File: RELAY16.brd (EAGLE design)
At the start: 118.1 x 69.8 mm, 118 parts, among them J1 Analog, J2 POWER, J3 Digital_0_7, J4 M100.1, J5 ICSPPTH, J6 Digital_0_7, J7 PWR SELECT, J8 Digital_0_7, J9 Digital_0_7, Q1 2N7002, Q10 2N7002, Q11 2N7002, Q12 2N7002, Q13 2N7002, Q14 2N7002, Q15 2N7002, Q16 2N7002, Q2 2N7002, Q3 2N7002, Q4 2N7002, Q5 2N7002, Q6 2N7002, Q7 2N7002, Q8 2N7002, Q9 2N7002

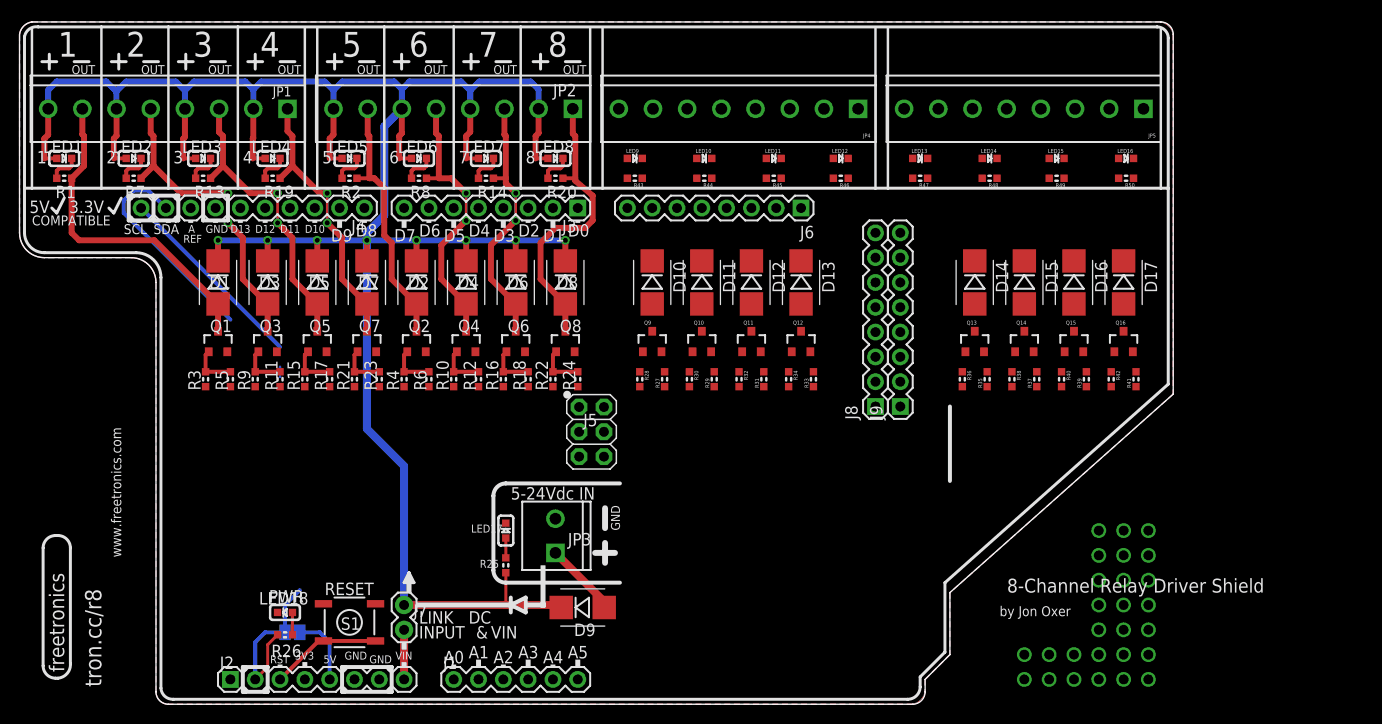
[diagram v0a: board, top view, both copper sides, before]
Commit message: Rough draft
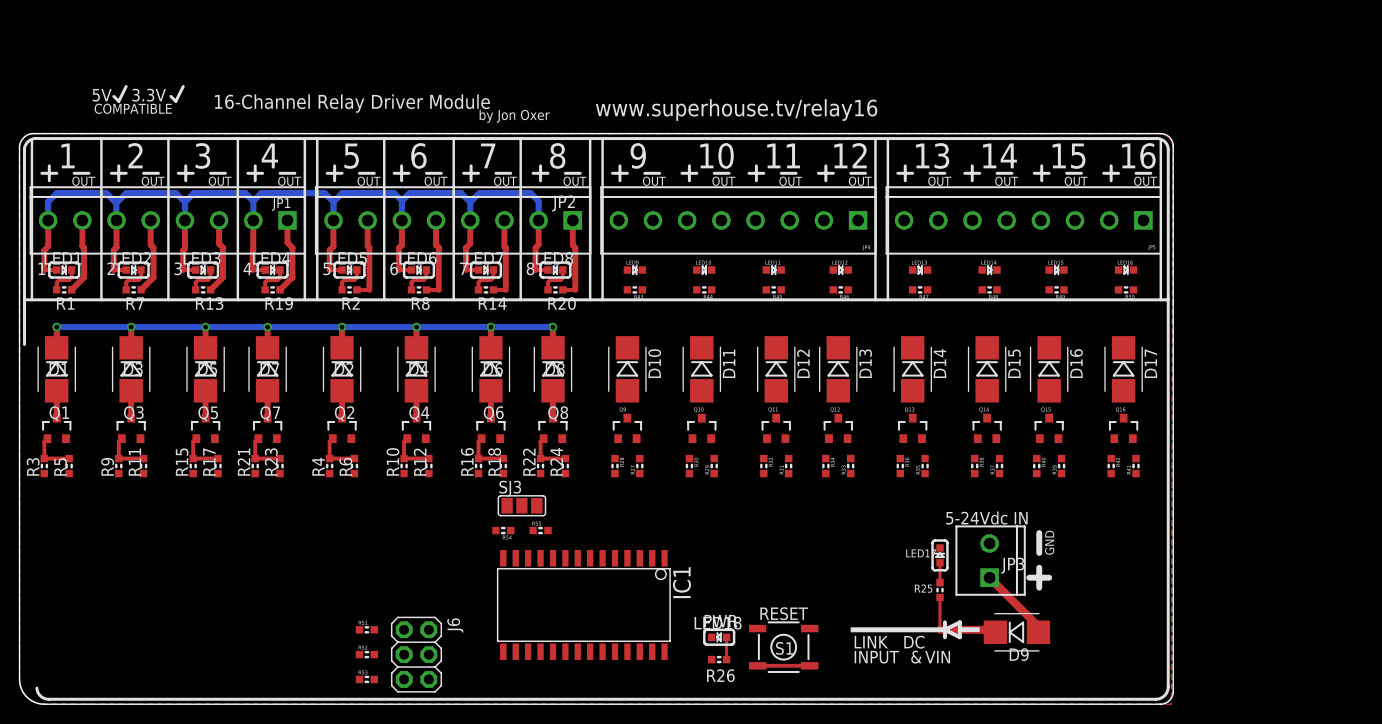
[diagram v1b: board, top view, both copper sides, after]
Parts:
- removed J1: Analog, freetronics:1X06
- removed J2: POWER, freetronics:1X08
- removed J3, J8, J9: Digital_0_7, freetronics:1X08
- removed J4: M100.1, freetronics-original:1X10
- removed J5: ICSPPTH, freetronics-jon:2X03PTH
- removed J7: PWR SELECT, SparkFun:1X02
- removed SJ4: (no value), freetronics-jon:SJ
- added IC1: MCP23017SO, microchip:SO28W
- added R51, R52, R53: 10K, freetronics-master-v1:0603
- added R54, R55: 4K7, freetronics-master-v1:0603
- added SJ3: (no value), freetronics-master-v1.1:SJ_2
- J6: value Digital_0_7 -> (none); device freetronics:1X08 -> freetronics-master-v1.1:2X03
- moved J6 60.3 mm to (40.6, 5.08), turned to 270 degrees
- moved D9 44.5 mm to (102.1, 7.37)
- moved LED18 44.5 mm to (71.6, 6.86)
- moved R26 44.5 mm to (71.6, 4.57)
- moved S1 44.5 mm to (78.2, 5.84)
- moved JP3 44.5 mm to (99.3, 13.0)
- moved LED17 44.5 mm to (94.2, 15.2)
- moved R25 44.5 mm to (94.2, 11.7)
- moved D1 18.8 mm to (3.81, 34.3)
- moved Q1 18.8 mm to (3.81, 28.2)
- moved R3 18.8 mm to (2.54, 24.4)
- moved R5 18.8 mm to (5.08, 24.4)
- moved Q3 16.6 mm to (11.4, 28.2)
- moved D3 16.6 mm to (11.4, 34.3)
- moved R11 16.6 mm to (12.7, 24.4)
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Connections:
- removed net 3V3: J2.4
- removed net 5V: J2.5, SJ4.2
- removed net A0: J1.1
- removed net A1: J1.2
- removed net A2: J1.3
- removed net A3: J1.4
- removed net A4_SDA: J1.5
- removed net A5_SCL: J1.6
- removed net AREF: J4.8
- removed net D0_RX: J3.1
- removed net D10: J4.3
- removed net D11_MOSI: J4.4
- removed net D12_MISO: J4.5
- removed net D13_SCK: J4.6
- removed net D1_TX: J3.2
- removed net D2: J3.3
- removed net D22: J8.8
- removed net D23: J9.8
- removed net D24: J8.7
- removed net D25: J9.7
- removed net D26: J8.6
- removed net D27: J9.6
- removed net D28: J8.5
- removed net D29: J9.5
- removed net D3: J3.4
- removed net D30: J8.4
- removed net D31: J9.4
- removed net D32: J8.3
- removed net D33: J9.3
- removed net D34: J8.2
- removed net D35: J9.2
- removed net D36: J8.1
- removed net D37: J9.1
- removed net D4: J3.5
- removed net D5: J3.6
- removed net D6: J3.7
- removed net D7: J3.8
- removed net D8: J4.1
- removed net D9: J4.2
- removed net N$71: J6.8
- removed net N$72: J6.7
- removed net N$73: J6.6
- removed net N$74: J6.5
- removed net N$75: J6.4
- removed net N$76: J6.3
- removed net N$77: J6.2
- removed net N$78: J6.1
- removed net NC: J2.1
- removed net R3_SCL: J4.10
- removed net R3_SDA: J4.9
- removed net VIN: J2.8, J7.2
- new net ADDR0: IC1.15, J6.2, R51.2
- new net ADDR1: IC1.16, J6.4, R52.2
- new net ADDR2: IC1.17, J6.6, R53.2
- new net GPB0: IC1.1, R28.2
- new net GPB1: IC1.2, R30.2
- new net GPB2: IC1.3, R32.2
- new net GPB3: IC1.4, R34.2
- new net GPB4: IC1.5, R36.2
- new net GPB5: IC1.6, R38.2
- new net GPB6: IC1.7, R40.2
- new net GPB7: IC1.8, R42.2
- new net N$2: R55.2, SJ3.3
- new net N$6: R54.2, SJ3.1
- new net SCL: IC1.12, R55.1
- new net SDA: IC1.13, R54.1
- net 12V: no longer J7.1
- net GND: now also IC1.10, R51.1, R52.1, R53.1; no longer J2.6, J2.7, J4.7
- net GPA0: now also IC1.21; no longer R28.2
- net GPA1: now also IC1.22; no longer R30.2
- net GPA2: now also IC1.23; no longer R32.2
- net GPA3: now also IC1.24; no longer R34.2
- net GPA4: now also IC1.25; no longer R36.2
- net GPA5: now also IC1.26; no longer R38.2
- net GPA6: now also IC1.27; no longer R40.2
- net GPA7: now also IC1.28; no longer R42.2
- net IOREF: now also IC1.9, J6.1, J6.3, J6.5, SJ3.2; no longer J2.2, SJ4.1
- net RESET: now also IC1.18; no longer J2.3
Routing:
- net 12V: track 248.3 -> 199.2 mm
- net N$3: track 35.6 -> 10.7 mm, vias 2 -> 0
- net N$5: track 34.4 -> 10.8 mm
- net N$9: track 33.6 -> 10.8 mm, vias 2 -> 0
- net R3_SDA: track 22.2 -> 0.00 mm
- net N$11: track 31.6 -> 10.8 mm, vias 2 -> 0
- net R3_SCL: track 20.1 -> 0.00 mm
- net N$15: track 31.0 -> 11.3 mm, vias 2 -> 0
- net N$19: track 30.1 -> 11.4 mm
- net N$17: track 29.5 -> 11.3 mm, vias 2 -> 0
- net IOREF: track 17.7 -> 0.00 mm
- net N$13: track 26.4 -> 11.2 mm
- net 5V: track 7.28 -> 0.00 mm
- net RESET: track 11.5 -> 5.77 mm
- net VIN: track 5.08 -> 0.00 mm
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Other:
- board size 118.1 x 69.8 mm -> 118.1 x 58.4 mm
- board text added: "10"
- board text added: "11"
- board text added: "12"
- board text added: "13"
- board text added: "14"
- board text added: "15"
- board text added: "16"
- board text added: "16-Channel Relay Driver Module"
- board text added: "9"
- board text added: "www.superhouse.tv/relay16"
- board text removed: "3V3"
- board text removed: "8-Channel Relay Driver Shield"
- board text removed: "A0"
- board text removed: "A1"
- board text removed: "A2"
- board text removed: "A3"
- board text removed: "A4"
- board text removed: "A5"
- board text removed: "IO"
- board text removed: "RST"
- board text removed: "freetronics"
- board text removed: "tron.cc/r8"
- board text removed: "www.freetronics.com"
